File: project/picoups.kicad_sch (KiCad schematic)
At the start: 21 parts, among them J1 Conn_02x20_Odd_Even, J2 Conn_01x02, J3 Conn_01x02, SW1 SW_Push

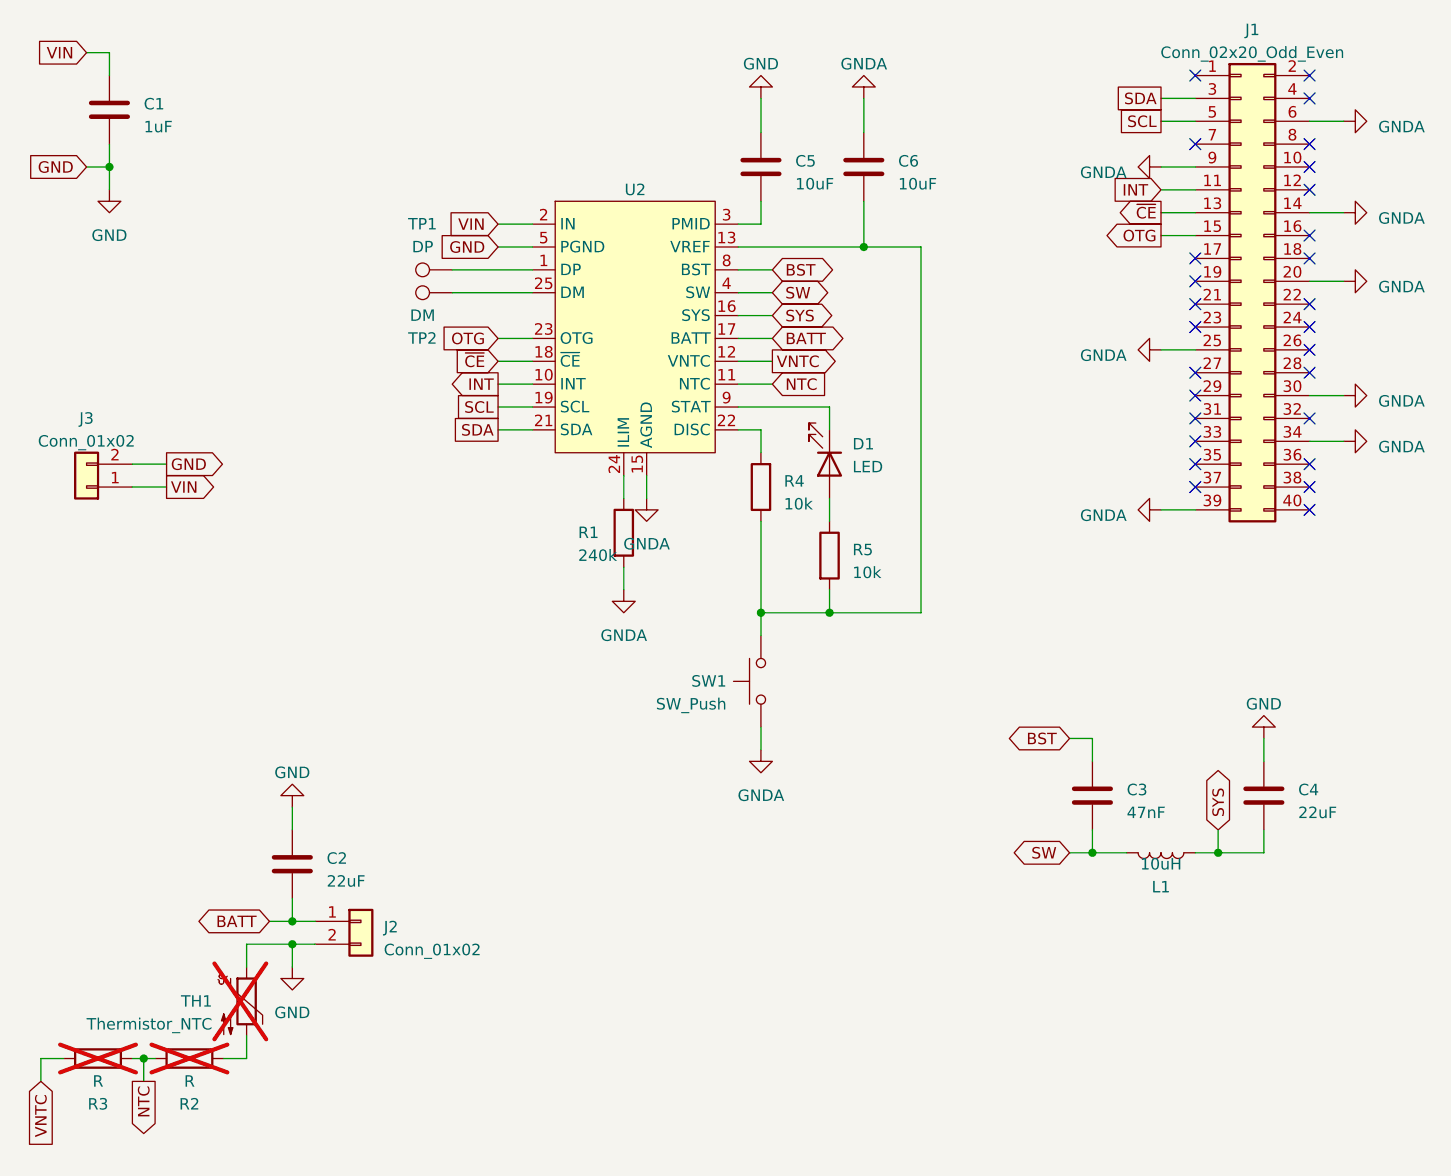
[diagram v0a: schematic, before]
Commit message: Cleanup
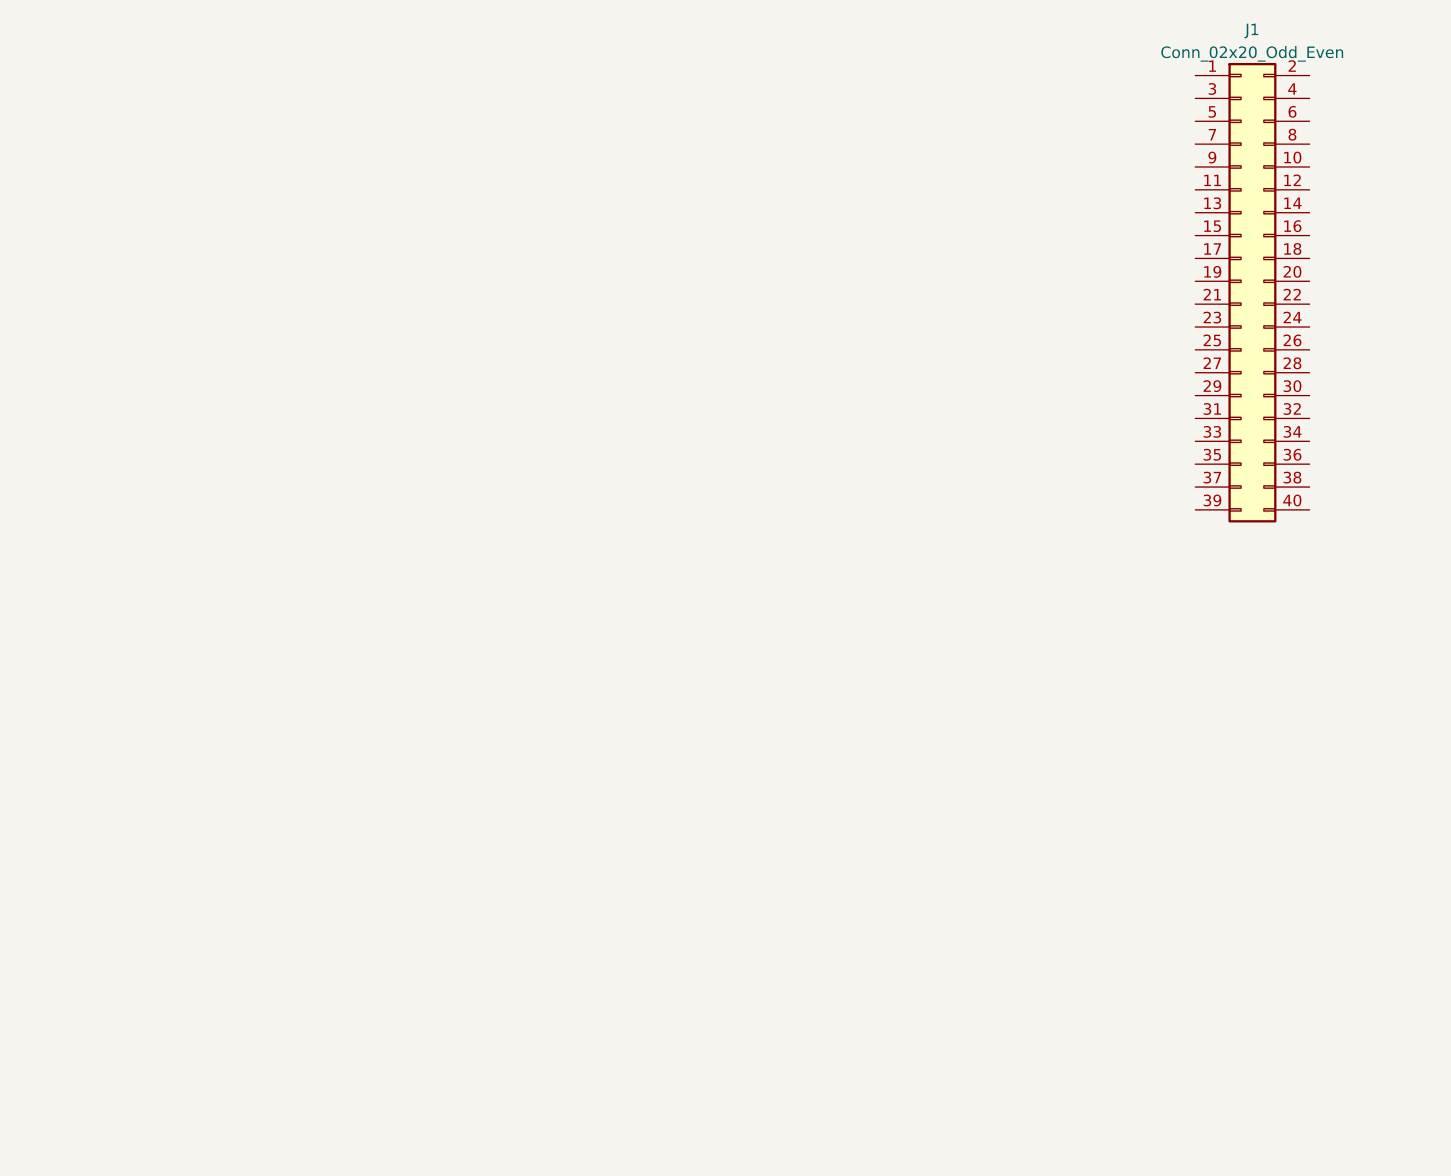
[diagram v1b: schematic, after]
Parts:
- removed C1: 1uF, Capacitor_SMD:C_0603_1608Metric, symbol Device:C
- removed C2, C4: 22uF, Capacitor_SMD:C_0805_2012Metric, symbol Device:C
- removed C3: 47nF, Capacitor_SMD:C_0603_1608Metric, symbol Device:C
- removed C5, C6: 10uF, Capacitor_SMD:C_0603_1608Metric, symbol Device:C
- removed D1: LED, LED_SMD:LED_0805_2012Metric, symbol Device:LED
- removed J2, J3: Conn_01x02, Connector_JST:JST_PH_S2B-PH-K_1x02_P2.00mm_Horizontal, symbol Connector_Generic:Conn_01x02
- removed L1: 10uH, PicoUPS:Inductor, symbol Device:L
- removed R1: 240k, Resistor_SMD:R_0201_0603Metric, symbol Device:R
- removed R2, R3: R, Resistor_SMD:R_0201_0603Metric, symbol Device:R
- removed R4, R5: 10k, Resistor_SMD:R_0201_0603Metric, symbol Device:R
- removed SW1: SW_Push, Button_Switch_SMD:SW_Push_1P1T_NO_Vertical_Wuerth_434133025816, symbol Switch:SW_Push
- removed TH1: Thermistor_NTC, Connector_PinHeader_2.54mm:PinHeader_1x02_P2.54mm_Vertical, symbol Device:Thermistor_NTC
- removed TP1: DP, TestPoint:TestPoint_Pad_D1.5mm, symbol Connector:TestPoint
- removed TP2: DM, TestPoint:TestPoint_Pad_D1.5mm, symbol Connector:TestPoint
- removed U2: ~, PicoUPS:MP2731, symbol PicoUPS:MP2731
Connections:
- removed net GNDA: J1.14 (Pin_14), J1.20 (Pin_20), J1.25 (Pin_25), J1.30 (Pin_30), J1.34 (Pin_34), J1.39 (Pin_39), J1.6 (Pin_6), J1.9 (Pin_9)
- net INT: no longer names the net of J1.11 (Pin_11)
- net OTG: no longer names the net of J1.15 (Pin_15)
- net SCL: no longer names the net of J1.5 (Pin_5)
- net SDA: no longer names the net of J1.3 (Pin_3)
- net ~{CE}: no longer names the net of J1.13 (Pin_13)
- no-connect marks 27 -> 0
